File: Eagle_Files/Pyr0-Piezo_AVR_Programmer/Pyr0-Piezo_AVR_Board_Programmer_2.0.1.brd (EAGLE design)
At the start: 42.6 x 46.5 mm, 71 parts, among them J2 FFC_MOLEX_0.5MM, U1 ATMEGA48/88/168/328PA, U4 LM2902QT

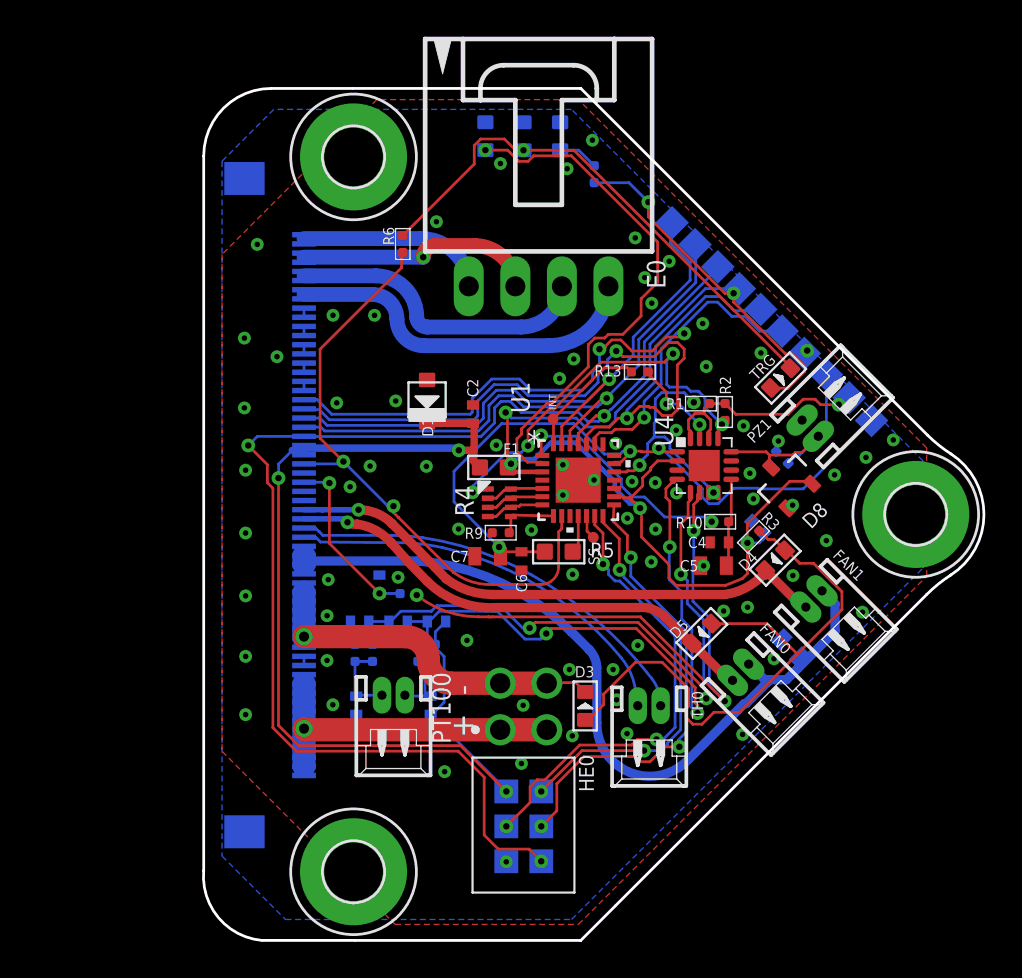
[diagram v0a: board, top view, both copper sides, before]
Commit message: sync all boards for Rev.2.0.1 before gerberization
- added test pads for debugging amp circuit
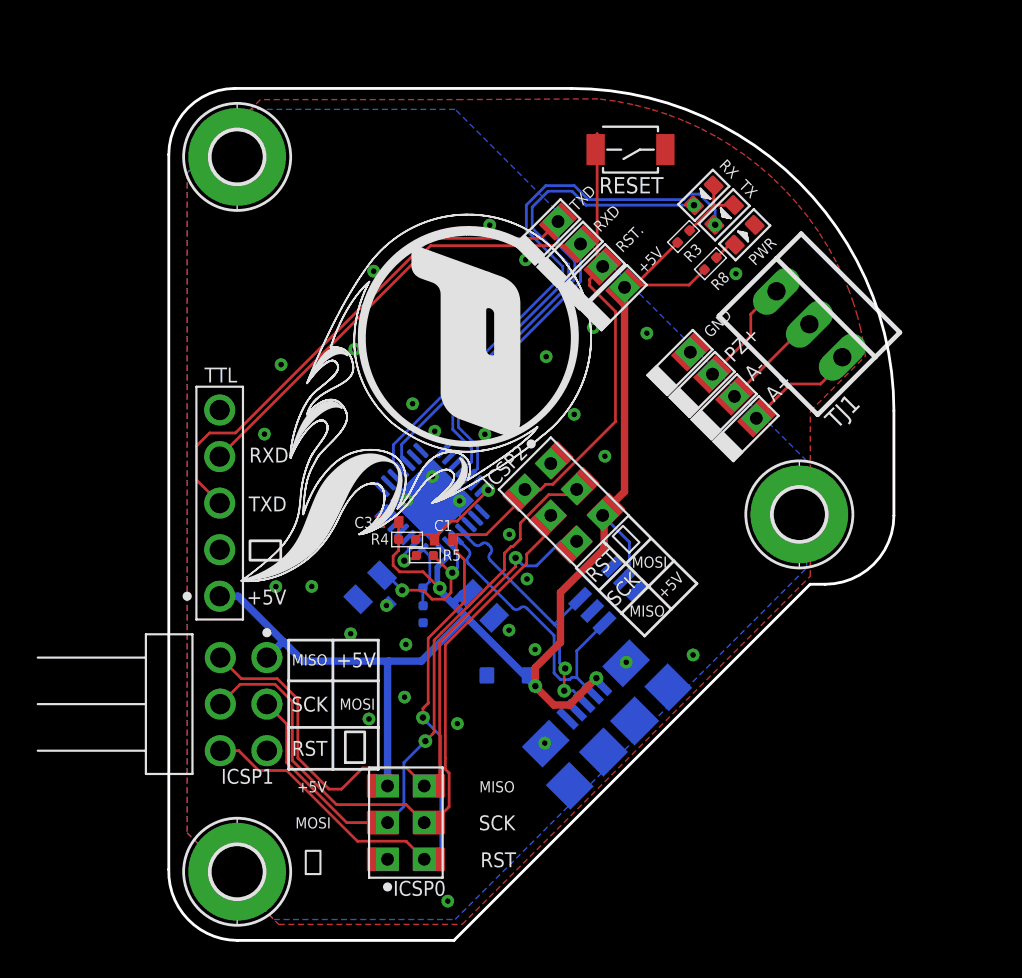
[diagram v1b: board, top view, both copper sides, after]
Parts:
- removed 5V, MISO, MOSI, RST, SCK: TPTP13SQ, PiezoFFC:TP13SQ
- removed C10, C11, C8, C9: 0.1uF, PiezoFFC:CAPC1005X50
- removed C12: 1uF, PiezoFFC:CAPC1005X50
- removed C13: 10nF, PiezoFFC:CAPC1005X50
- removed C6: 10uF, PiezoFFC:CAPC1005X50
- removed C7: 3.3uF, PiezoFFC:CAPC1609X80
- removed D1: ZENER_DIODE_PLZ5V1C, PiezoFFC:DO-219AC
- removed D4, D5, ERR, RDY, TRG: (no value), PiezoFFC:SEEED-LED_LED-0603
- removed D8: BAV199, PiezoFFC:SOT23
- removed E0: C-GRID-04-70553, PiezoFFC:70553-04
- removed F1: 500mA, PiezoFFC:SEEED-RESISTOR_R0603
- removed FAN0, FAN1, PT100, PZ1, TH0: CON-MOLEX-2P-1.27MM048, PiezoFFC:53048-02
- removed HE0: JST-2.54-2X2JST-DUPONT-2.54-2X2, PiezoFFC:HDRRAR4W64P254_2X2_556X736X556B
- removed INT, SS: TPTP06R, testpad:TP06R
- removed J2: FFC_MOLEX_0.5MM, PiezoFFC:FFC-60P_0.5_MOLEX_505110-6091
- removed R10, R11, R7: 10K, PiezoFFC:R0402
- removed R12, R14: 2K2, PiezoFFC:R0402
- removed R13, R15: 100R, PiezoFFC:R0402
- removed R19: 1M, PiezoFFC:R0402
- removed R6: 4.7k, PiezoFFC:R0402
- removed R9: 1K, PiezoFFC:R0402
- removed SCL, SDA, ⏚: TPTP13SQ, testpad:TP13SQ
- removed U4: LM2902QT, PiezoFFC:QFN16
- added D2: TVS_DIODE_CM1293A, PiezoFFC:SC-74-6
- added ICSP0, ICSP2: ICSP_HEADERSPRING_3.48X1.1, PiezoFFC:ICSP_3X2_3.48X1.1_SPRING_CONTACTS
- added ICSP1: ICSP_HEADERICSP_2.54MM_RIGHT, PiezoFFC:ICSP_2X3_2.54_RIGHT
- added J1: 10118192-0001LF, PiezoFFC:AMPHENOL_10118192-0001LF
- added RESET: (no value), PiezoFFC:SEEED-SWITCH_SW2-2.6-3.0X2.5X1.2+0.4MM
- added RX, TX: (no value), PiezoFFC:SEEED-LED_LED-0603
- added TJ1: 22-23-2031, con-molex:22-23-2031
- added TTL: JST-2.54MM_5P-2.54JST_2.54MM_5P_F, PiezoFFC:HDRVR5W64P254_1X5_1270X254X575B
- +5V, GND, RST., RXD, TXD: value TPTP13SQ -> TPSPRING_CONTACT_3.5X1.1; device testpad:TP13SQ -> PiezoFFC:SPRING_CONTACT_3.48X1.10
- A+, A-, PZ+: value TPTP13SQ -> TPSPRING_CONTACT_3.5X1.1; device PiezoFFC:TP13SQ -> PiezoFFC:SPRING_CONTACT_3.48X1.10
- C3: value 1uF -> 0.1uF; device PiezoFFC:CAPC1609X80 -> PiezoFFC:CAPC1005X50
- C4: value 10uF -> 4.7uF; device PiezoFFC:CAPC1005X50 -> PiezoFFC:CAPC2012X130
- C5: value 3.3uF -> 4.7uF; device PiezoFFC:CAPC1609X80 -> PiezoFFC:CAPC2012X130
- D3: value (none) -> ZENER_DIODE_PLZ5V1C; device PiezoFFC:SEEED-LED_LED-0603 -> PiezoFFC:DO-219AC
- H1, H2, H3: value HOLES_MOUNT-PAD-ROUND3.2 -> HOLES_MOUNT-PAD-ROUND2.8; device PiezoFFC:HOLES_3,2-PAD -> PiezoFFC:HOLES_2,8-PAD
- R1: value 1M -> 22K
- R2: value 10K -> 47K
- R3, R8: value 1K -> (none)
- R4: value 1K -> 10K; device PiezoFFC:EXBN8V -> PiezoFFC:R0402
- R5: device PiezoFFC:SEEED-RESISTOR_R0603 -> PiezoFFC:R0402
- U1: value ATMEGA48/88/168/328PA -> CP2102N-A01-GQFN28; device PiezoFFC:28M1 -> PiezoFFC:QFN50P500X500X80-29N
- moved C3 22.9 mm to (12.0, 23.0), flipped to the top, turned to 0 degrees
- moved R2 19.8 mm to (13.9, 17.9), flipped to the bottom
- moved C5 18.8 mm to (11.0, 19.4), flipped to the bottom, turned to 315 degrees
- moved R1 17.8 mm to (14.3, 19.4), flipped to the bottom, turned to 270 degrees
- moved C1 17.1 mm to (15.0, 22.0), flipped to the top, turned to 180 degrees
- moved R3 16.8 mm to (28.1, 38.5)
- moved C4 13.4 mm to (17.1, 18.4), flipped to the bottom, turned to 225 degrees
- moved PWR 11.4 mm to (31.4, 38.6), flipped to the top, turned to 45 degrees
- moved C2 10.8 mm to (12.4, 18.9), flipped to the bottom, turned to 135 degrees
- moved U$1 9.60 mm to (16.4, 33.0), flipped to the top, turned to 270 degrees
- moved A+ 9.04 mm to (29.7, 31.0), flipped to the top, turned to 225 degrees
- moved U1 8.05 mm to (14.4, 24.1), flipped to the bottom, turned to 45 degrees
- moved R8 8.00 mm to (29.6, 37.1), flipped to the top, turned to 135 degrees
- moved R5 7.31 mm to (14.0, 21.1)
- moved H1 6.35 mm to (3.73, 3.87)
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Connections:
- net N$2 renamed PWR_IND
- removed net +5V: +5V.TP, C1.1, D8.2, F1.2, R3.1, R8.1, TRG.+, U1.16, U1.3, U4.2
- removed net E0_1A: E0.2, J2.57, J2.58
- removed net E0_1B: E0.1, J2.59, J2.60
- removed net E0_2A: E0.3, J2.55, J2.56
- removed net E0_2B: E0.4, J2.53, J2.54
- removed net ERR_LED: ERR.+, U1.2
- removed net FAN0_GATE: D5.-, FAN0.1, J2.29
- removed net FAN1_GATE: D4.-, FAN1.1, J2.30
- removed net GADJ_R0: R4.2, R4.8, U1.5
- removed net GADJ_R1: R4.3, R4.7, U1.6
- removed net GADJ_R2: R4.4, R4.6, U1.7
- removed net GADJ_R3: R4.5, R9.2, U1.8
- removed net GAIN_FB: R2.1, R4.1, U4.13
- removed net GAIN_OUT: A-.TP, R1.2, R2.2, U4.14, U4.16
- removed net HE0-: D3.-, HE0.3, HE0.4, J2.15, J2.16, J2.17, J2.18, J2.19, J2.20, J2.21, J2.22
- removed net PT100+: C8.1, PT100.2, R12.1, R7.2
- removed net PT100-: C9.2, PT100.1, R11.2, R14.2
- removed net PT100_AMP+: C10.1, C12.2, R7.1, U4.4
- removed net PT100_AMP-: C11.2, C12.1, R11.1, U4.5
- removed net PT100_OUT: C13.2, J2.33, R15.1
- removed net PT100_R: R15.2, U4.6
- removed net PZ+: D8.3, PZ+.TP, PZ1.1, R19.2, U4.12
- removed net PZ_AMP_OUT: R13.1, U4.15
- removed net SCL: J2.41, SCL.TP, U1.24
- removed net SDA: J2.42, SDA.TP, U1.23
- removed net SPI_SS: SS.TP, U1.12
- removed net TH0+: J2.27, TH0.1
- removed net TH0-: J2.28, TH0.2
- removed net TRG_LED: R6.2, RDY.+, TRG.-
- removed net TTL_RXD: J2.39, RXD.TP, U1.26
- removed net TTL_TXD: J2.40, TXD.TP, U1.27
- removed net VCC: HE0.1, HE0.2, J2.1, J2.10, J2.11, J2.12, J2.2, J2.3, J2.4, J2.5, J2.6, J2.7, J2.8, J2.9
- removed net VCC_REG: 5V.TP, C10.2, C2.2, C8.2, D1.P$2, F1.1, J2.36, J2.37, R12.2
- removed net VCOMP_PWM: R5.2, U1.11
- removed net VCOMP_SENSE: A+.TP, C6.2, C7.2, R5.1, U1.20, U4.1
- removed net VREF_IN: C4.2, C5.2, R10.1, U4.9
- removed net V_FOL_PWM: R10.2, U1.1
- removed net V_FOL_SENSE: R1.1, U1.19, U4.7, U4.8
- removed net V_INT: C3.1, FAN0.2, FAN1.2, J2.23, J2.24, J2.25, J2.26
- removed net X_1A: J2.47, J2.48
- removed net X_1B: J2.49, J2.50
- removed net X_2A: J2.45, J2.46
- removed net X_2B: J2.43, J2.44
- removed net X_MIN_TRIG: J2.34
- removed net Z_MIN_TRIG: J2.35, R6.1, U1.9
- removed net Z_TRG: INT.TP, R13.2, U1.28
- new net 5V_DC: +5V.TH, +5V.TP, C3.2, C4.1, D2.5, D3.P$2, ICSP0.5, ICSP0.P$5, ICSP1.1, ICSP2.5, ICSP2.P$5, J1.1, R1.2, R3.1, R4.1, R8.1, TTL.1, TTL.5, U1.7
- new net D+: D2.3, J1.3, U1.4
- new net D-: D2.1, J1.2, U1.5
- new net N$1: PZ+.TH, PZ+.TP, TJ1.3
- new net N$2: A-.TH, A-.TP, TJ1.2
- new net N$3: A+.TH, A+.TP, TJ1.1
- new net PGM_RST: C1.2, R4.2, U1.28
- new net RST_PULLUP: R5.1, U1.9
- new net RXD: RXD.TH, RXD.TP, TTL.4, U1.26
- new net RXT: RX.-, U1.19
- new net TXD: TTL.3, TXD.TH, TXD.TP, U1.25
- new net TXT: TX.-, U1.18
- new net VBUS: R1.1, R2.2, U1.8
- new net VDD: C2.2, C5.1, R5.2, U1.6
- net GND: now also C3.1, C4.2, C5.2, D2.2, D3.P$1, GND.TH, H1.B2,8, H2.B2,8, H3.B2,8, ICSP0.1, ICSP0.P$1, ICSP1.3, ICSP2.1, ICSP2.P$1, J1.5, J1.SH1, J1.SH2, J1.SH3, J1.SH4, J1.SH5, J1.SH6, R2.1, RESET.1, TTL.2, U1.3; no longer C1.2, C11.1, C13.1, C3.2, C4.1, C5.1, C6.1, C7.1, C9.1, D1.P$1, D8.1, ERR.-, H1.B3,2, H2.B3,2, H3.B3,2, J2.13, J2.14, J2.31, J2.32, J2.51, J2.52, J2.S$1, J2.S$2, PZ1.2, R14.1, R19.1, R9.1, RDY.-, U1.18, U1.4, U4.11, ⏚.TP
- net LED_VCC: now also RX.+, TX.+; no longer D3.+, D4.+, D5.+
- net RST: now also C1.1, ICSP0.2, ICSP0.P$2, ICSP1.4, ICSP2.2, ICSP2.P$2, RESET.2, RST..TH; no longer J2.38, RST.TP, U1.25
- net SPI_MISO: now also ICSP0.6, ICSP0.P$6, ICSP1.6, ICSP2.6, ICSP2.P$6; no longer MISO.TP, U1.14
- net SPI_MOSI: now also ICSP0.4, ICSP0.P$4, ICSP1.2, ICSP2.4, ICSP2.P$4; no longer MOSI.TP, U1.13
- net SPI_SCK: now also ICSP0.3, ICSP0.P$3, ICSP1.5, ICSP2.3, ICSP2.P$3; no longer SCK.TP, U1.15
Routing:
- net 5V_DC: track 0.00 -> 83.4 mm, vias 0 -> 3
- net +5V: track 74.4 -> 0.00 mm, vias 6 -> 0
- net VCC_REG: track 56.6 -> 0.00 mm, vias 3 -> 0
- net SCL: track 46.2 -> 0.00 mm, vias 2 -> 0
- net TXD: track 0.00 -> 45.8 mm
- net V_INT: track 43.3 -> 0.00 mm
- net SDA: track 41.6 -> 0.00 mm, vias 3 -> 0
- net RXD: track 0.00 -> 40.6 mm
- net VCOMP_SENSE: track 38.6 -> 0.00 mm, vias 3 -> 0
- net PT100_AMP+: track 34.9 -> 0.00 mm, vias 3 -> 0
- net PT100_AMP-: track 34.7 -> 0.00 mm, vias 3 -> 0
- net TTL_TXD: track 34.3 -> 0.00 mm, vias 1 -> 0
- net Z_MIN_TRIG: track 33.9 -> 0.00 mm, vias 2 -> 0
- net TTL_RXD: track 32.2 -> 0.00 mm, vias 1 -> 0
- net TXT: track 0.00 -> 31.7 mm, vias 0 -> 1
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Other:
- board size 42.6 x 46.5 mm -> 39.6 x 46.5 mm
- board text added: "+5V"
- board text added: "A+"
- board text added: "A-"
- board text added: "MISO"
- board text added: "MOSI"
- board text added: "PZ+"
- board text added: "RST"
- board text added: "RXD"
- board text added: "SCK"
- board text added: "TXD"
- board text added: "⏚"
- board text removed: "+ -"
- board text removed: "2B 2A 1A 1B"
- board text removed: "Fan0"
- board text removed: "Fan1"
- board text removed: "HE0"
- board text removed: "PZ1"
- board text removed: "TH0"
